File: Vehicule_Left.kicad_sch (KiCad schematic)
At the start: 16 parts, among them Q19 IRLZ44N, U4 LM339

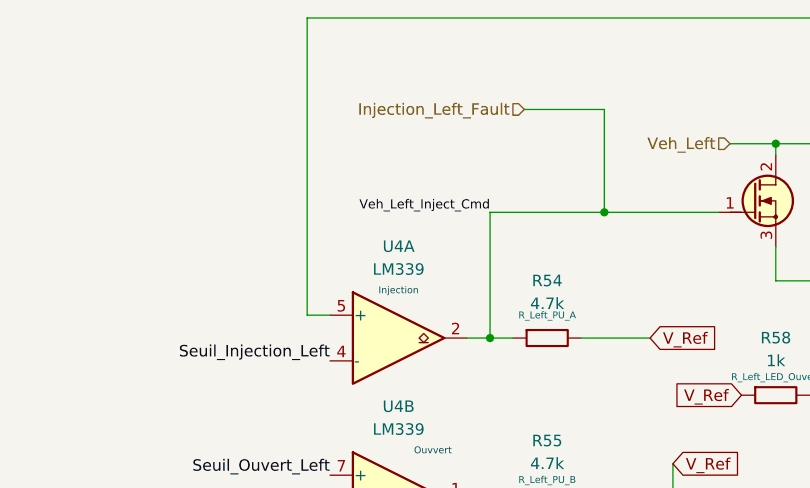
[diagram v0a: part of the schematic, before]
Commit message: Add files via upload
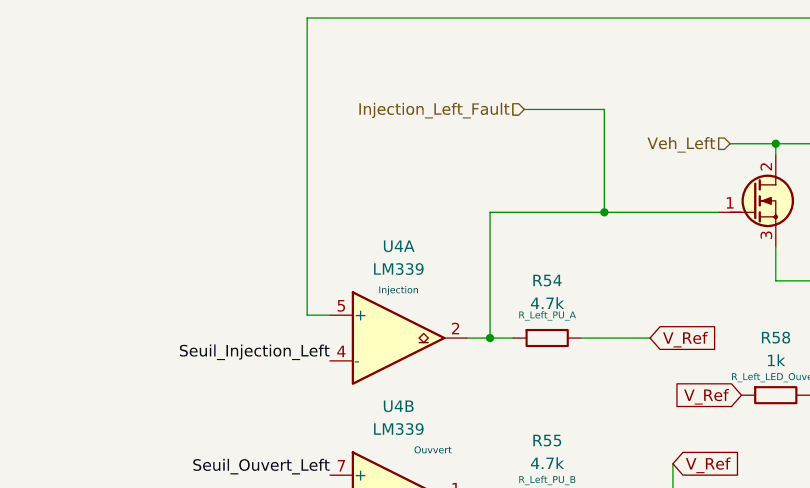
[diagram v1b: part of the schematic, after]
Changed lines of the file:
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@@
-		)
-	)
-	(label "Veh_Left_Inject_Cmd"
-		(at 86.36 39.37 180)
-		(effects
-			(font
-				(size 1.016 1.016)
-			)
-			(justify right bottom)
 		)
 	)
